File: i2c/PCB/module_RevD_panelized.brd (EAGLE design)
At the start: 100 x 100 mm, 786 parts, among them IC1 ATTINY85-20SU, IC2 ATTINY85-20SU, IC3 ATTINY85-20SU, IC4 ATTINY85-20SU, IC5 ATTINY85-20SU, IC6 ATTINY85-20SU, J1 M20-9980346, J2 M20-9980346, J3 M20-9980346, J4 M20-9980346, J5 M20-9980346, J6 M20-9980346

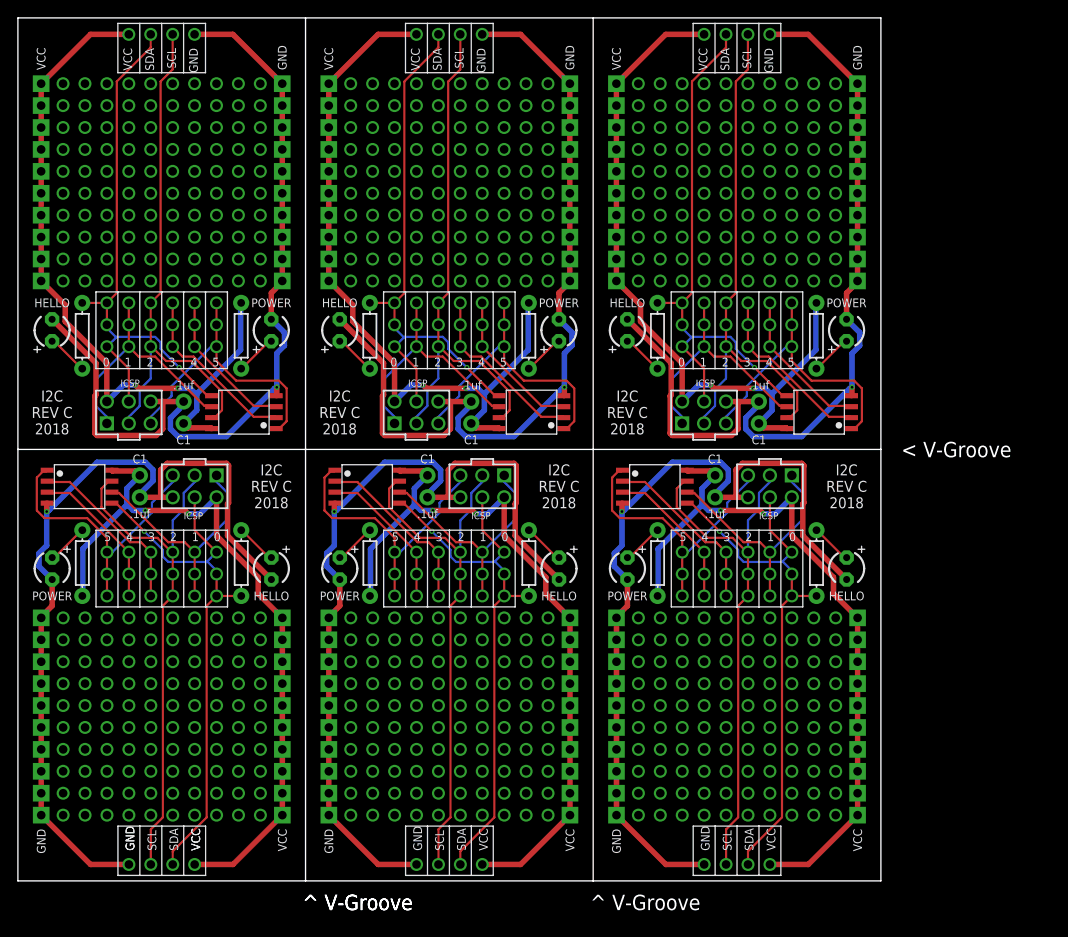
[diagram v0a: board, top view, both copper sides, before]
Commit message: Rework of revD boards
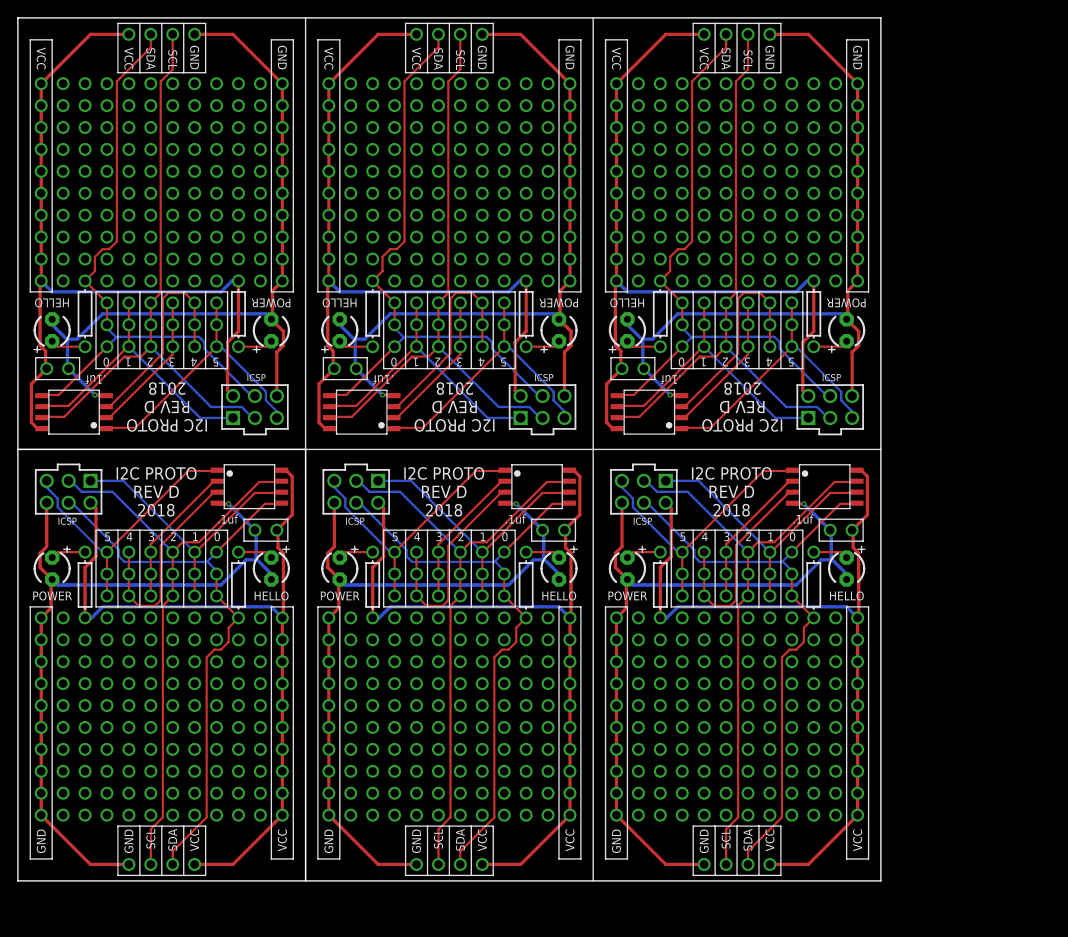
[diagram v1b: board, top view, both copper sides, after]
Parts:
- removed GND, GND1, GND2, GND3, GND4, GND5, VCC, VCC1, VCC2, VCC3, VCC4, VCC5: 10X-PADS, BadgeParts:10X-PADS
- removed R1, R10, R11, R12, R2, R3, R4, R5, R6, R7, R8, R9: 220, SparkFun-Resistors:AXIAL-0.3
- added U$739, U$740, U$741, U$742, U$743, U$744, U$745, U$746, U$747, U$748, U$749, U$750, U$751, U$752, U$753, U$754, U$755, U$756, U$757, U$758, U$759, U$760, U$761, U$762, U$763, U$764, U$765, U$766, U$767, U$768, U$769, U$770, U$771, U$772, U$773, U$774, U$775, U$776, U$777, U$778, U$779, U$780, U$781, U$782, U$783, U$784, U$785, U$790, U$791, U$792, U$793, U$794, U$795, U$796, U$797, U$798, U$799, U$800, U$801, U$802, U$803, U$804, U$805, U$806, U$807, U$808, U$809, U$810, U$811, U$812, U$813, U$814, U$815, U$816, U$817, U$818, U$819, U$820, U$821, U$822, U$823, U$824, U$825, U$826, U$827, U$828, U$829, U$830, U$831, U$832, U$833, U$834, U$835, U$839, U$840, U$841, U$842, U$843, U$844, U$845, U$846, U$847, U$848, U$849, U$850, U$851, U$852, U$853, U$854, U$855, U$856, U$857, U$858: ONE_PAD, BadgeParts:1X01
- added U$786: GND, BadgeParts:1X01
- added U$787: VCC, BadgeParts:1X01
- added U$788: SDA, BadgeParts:1X01
- added U$789: SCL, BadgeParts:1X01
- added U$836: DECOUPLING_CAP, BadgeParts:DECOUPLING_CAP
- added U$837, U$838: RESISTOR, BadgeParts:AXIAL-0.3
- U$126, U$127, U$265, U$266, U$408, U$409, U$551, U$552, U$694, U$695: value ONE_PAD -> RESISTOR; device BadgeParts:1X01 -> BadgeParts:AXIAL-0.3
- U$194, U$317, U$440, U$563, U$686: value GND -> ONE_PAD
- U$195, U$318, U$441, U$564, U$687: value VCC -> ONE_PAD
- U$196, U$319, U$442, U$565, U$688: value SDA -> ONE_PAD
- U$197, U$320, U$443, U$566, U$689: value SCL -> ONE_PAD
- U$214, U$357, U$500, U$643: value ONE_PAD -> GND
- U$215, U$358, U$501, U$644: value ONE_PAD -> VCC
- U$216, U$359, U$502, U$645: value ONE_PAD -> SDA
- U$217, U$360, U$503, U$646: value ONE_PAD -> SCL
- U$246, U$369, U$492, U$615, U$738: value DECOUPLING_CAP -> ONE_PAD; device BadgeParts:DECOUPLING_CAP -> BadgeParts:1X01
- U$264, U$407, U$550, U$693: value ONE_PAD -> DECOUPLING_CAP; device BadgeParts:1X01 -> BadgeParts:DECOUPLING_CAP
- moved U$428 121.6 mm to (97.3, 7.62), turned to 0 degrees
- moved U$424 116.1 mm to (97.3, 12.7), turned to 0 degrees
- moved U$426 111.8 mm to (97.3, 10.2), turned to 0 degrees
- moved U$420 111.0 mm to (97.3, 17.8), turned to 0 degrees
- moved U$422 110.7 mm to (97.3, 15.2), turned to 0 degrees
- moved U$425 109.8 mm to (97.3, 25.4), turned to 0 degrees
- moved U$429 107.4 mm to (97.3, 20.3), turned to 0 degrees
- moved U$427 106.9 mm to (97.3, 22.9), turned to 0 degrees
- moved U$421 105.3 mm to (97.3, 30.5), turned to 0 degrees
- moved U$71 104.5 mm to (12.9, 1.91), turned to 180 degrees
- moved U$423 104.2 mm to (97.3, 27.9), turned to 0 degrees
- moved U$73 102.7 mm to (15.4, 1.91), turned to 0 degrees
- moved U$8 101.7 mm to (5.24, 7.62), turned to 0 degrees
- moved U$72 101.0 mm to (17.9, 1.91), turned to 0 degrees
- moved U$74 99.6 mm to (20.5, 1.91), turned to 90 degrees
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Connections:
- removed net GND4: GND4.P$1, GND4.P$10, GND4.P$2, GND4.P$3, GND4.P$4, GND4.P$5, GND4.P$6, GND4.P$7, GND4.P$8, GND4.P$9, HELLO4.NEG, IC5.GND, J5.GND, POWER4.NEG, U$563.P$1, U$615.1
- removed net GND5: GND5.P$1, GND5.P$10, GND5.P$2, GND5.P$3, GND5.P$4, GND5.P$5, GND5.P$6, GND5.P$7, GND5.P$8, GND5.P$9, HELLO5.NEG, IC6.GND, J6.GND, POWER5.NEG, U$686.P$1, U$738.1
- removed net PB28: IC5.PB5, J5.5/RST, U$582.P$1, U$583.P$1, U$584.P$1
- removed net PB29: IC5.PB1, J5.1/MISO, U$570.P$1, U$571.P$1, U$572.P$1
- removed net PB34: IC6.PB5, J6.5/RST, U$705.P$1, U$706.P$1, U$707.P$1
- removed net PB35: IC6.PB1, J6.1/MISO, U$693.P$1, U$694.P$1, U$695.P$1
- new net GND6: HELLO4.NEG, IC5.GND, J5.GND, POWER4.NEG, U$643.P$1, U$693.P$1, U$696.P$1, U$697.P$1, U$698.P$1, U$699.P$1, U$700.P$1, U$701.P$1, U$702.P$1, U$703.P$1, U$704.P$1, U$705.P$1
- new net GND7: HELLO5.NEG, IC6.GND, J6.GND, POWER5.NEG, U$786.P$1, U$836.P$1, U$839.P$1, U$840.P$1, U$841.P$1, U$842.P$1, U$843.P$1, U$844.P$1, U$845.P$1, U$846.P$1, U$847.P$1, U$848.P$1
- new net PB36: IC6.PB4, U$802.P$1, U$803.P$1, U$804.P$1
- new net PB37: IC6.PB2, J6.2/SCK/SCL, U$789.P$1, U$796.P$1, U$797.P$1, U$798.P$1
- new net PB38: IC6.PB5, J6.5/RST, U$805.P$1, U$806.P$1, U$807.P$1
- new net PB39: IC6.PB1, J6.1/MISO, U$793.P$1, U$794.P$1, U$795.P$1
- net GND: now also U$100.P$1, U$123.P$1, U$124.P$1, U$125.P$1, U$128.P$1, U$129.P$1, U$130.P$1, U$131.P$1, U$132.P$1, U$133.P$1, U$99.P$1; no longer GND.P$1, GND.P$10, GND.P$2, GND.P$3, GND.P$4, GND.P$5, GND.P$6, GND.P$7, GND.P$8, GND.P$9, U$123.1
- net GND1: now also U$214.P$1, U$264.P$1, U$267.P$1, U$268.P$1, U$269.P$1, U$270.P$1, U$271.P$1, U$272.P$1, U$273.P$1, U$274.P$1, U$275.P$1, U$276.P$1; no longer GND1.P$1, GND1.P$10, GND1.P$2, GND1.P$3, GND1.P$4, GND1.P$5, GND1.P$6, GND1.P$7, GND1.P$8, GND1.P$9, U$194.P$1, U$246.1
- net GND2: now also U$357.P$1, U$407.P$1, U$410.P$1, U$411.P$1, U$412.P$1, U$413.P$1, U$414.P$1, U$415.P$1, U$416.P$1, U$417.P$1, U$418.P$1, U$419.P$1; no longer GND2.P$1, GND2.P$10, GND2.P$2, GND2.P$3, GND2.P$4, GND2.P$5, GND2.P$6, GND2.P$7, GND2.P$8, GND2.P$9, U$317.P$1, U$369.1
- net GND3: now also U$500.P$1, U$550.P$1, U$553.P$1, U$554.P$1, U$555.P$1, U$556.P$1, U$557.P$1, U$558.P$1, U$559.P$1, U$560.P$1, U$561.P$1, U$562.P$1; no longer GND3.P$1, GND3.P$10, GND3.P$2, GND3.P$3, GND3.P$4, GND3.P$5, GND3.P$6, GND3.P$7, GND3.P$8, GND3.P$9, U$440.P$1, U$492.1
- net N$1: now also U$126.P$3; no longer R1.P$1
- net N$10: now also U$695.P$3; no longer R10.P$1
- net N$11: now also U$837.P$3; no longer R11.P$1
- net N$12: now also U$838.P$3; no longer R12.P$1
- net N$2: now also HELLO.POS, U$127.P$3; no longer POWER1.POS, R3.P$1
- net N$3: now also POWER1.POS, U$265.P$3; no longer HELLO.POS, R2.P$1
- net N$4: now also U$266.P$3; no longer R4.P$1
- net N$5: now also U$408.P$3; no longer R5.P$1
- net N$6: now also U$409.P$3; no longer R6.P$1
- net N$7: now also U$551.P$3; no longer R7.P$1
- net N$8: now also U$552.P$3; no longer R8.P$1
- net N$9: now also U$694.P$3; no longer R9.P$1
- net PB0: now also U$127.P$4; no longer R2.P$2
- net PB10: now also U$233.P$1, U$234.P$1, U$235.P$1; no longer U$213.P$1, U$214.P$1, U$215.P$1
- net PB11: now also U$221.P$1, U$222.P$1, U$223.P$1; no longer U$201.P$1, U$202.P$1, U$203.P$1
- net PB12: now also U$359.P$1, U$361.P$1, U$362.P$1, U$363.P$1, U$409.P$4; no longer R6.P$2, U$319.P$1, U$321.P$1, U$322.P$1, U$323.P$1
- net PB13: now also U$370.P$1, U$371.P$1, U$372.P$1; no longer U$330.P$1, U$331.P$1, U$332.P$1
- net PB14: now also U$373.P$1, U$374.P$1, U$375.P$1; no longer U$333.P$1, U$334.P$1, U$335.P$1
- net PB15: now also U$360.P$1, U$367.P$1, U$368.P$1, U$369.P$1; no longer U$320.P$1, U$327.P$1, U$328.P$1, U$329.P$1
- net PB16: now also U$376.P$1, U$377.P$1, U$378.P$1; no longer U$336.P$1, U$337.P$1, U$338.P$1
- net PB17: now also U$364.P$1, U$365.P$1, U$366.P$1; no longer U$324.P$1, U$325.P$1, U$326.P$1
- net PB18: now also U$502.P$1, U$504.P$1, U$505.P$1, U$506.P$1, U$552.P$4; no longer R8.P$2, U$442.P$1, U$444.P$1, U$445.P$1, U$446.P$1
- net PB19: now also U$513.P$1, U$514.P$1, U$515.P$1; no longer U$453.P$1, U$454.P$1, U$455.P$1
- net PB20: now also U$516.P$1, U$517.P$1, U$518.P$1; no longer U$456.P$1, U$457.P$1, U$458.P$1
- net PB21: now also U$503.P$1, U$510.P$1, U$511.P$1, U$512.P$1; no longer U$443.P$1, U$450.P$1, U$451.P$1, U$452.P$1
- net PB22: now also U$519.P$1, U$520.P$1, U$521.P$1; no longer U$459.P$1, U$460.P$1, U$461.P$1
- net PB23: now also U$507.P$1, U$508.P$1, U$509.P$1; no longer U$447.P$1, U$448.P$1, U$449.P$1
- net PB24: now also U$645.P$1, U$647.P$1, U$648.P$1, U$649.P$1, U$695.P$4; no longer R10.P$2, U$565.P$1, U$567.P$1, U$568.P$1, U$569.P$1
- net PB25: now also U$656.P$1, U$657.P$1, U$658.P$1; no longer U$576.P$1, U$577.P$1, U$578.P$1
- net PB26: now also U$659.P$1, U$660.P$1, U$661.P$1; no longer U$579.P$1, U$580.P$1, U$581.P$1
- net PB27: now also U$646.P$1, U$653.P$1, U$654.P$1, U$655.P$1; no longer U$566.P$1, U$573.P$1, U$574.P$1, U$575.P$1
- net PB30: now also IC5.PB5, J5.5/RST, U$662.P$1, U$663.P$1, U$664.P$1; no longer IC6.PB0, J6.0/MOSI/SDA, R12.P$2, U$688.P$1, U$690.P$1, U$691.P$1, U$692.P$1
- net PB31: now also IC5.PB1, J5.1/MISO, U$650.P$1, U$651.P$1, U$652.P$1; no longer IC6.PB3, U$699.P$1, U$700.P$1, U$701.P$1
- net PB32: now also IC6.PB0, J6.0/MOSI/SDA, U$788.P$1, U$790.P$1, U$791.P$1, U$792.P$1, U$838.P$4; no longer IC6.PB4, U$702.P$1, U$703.P$1, U$704.P$1
- net PB33: now also IC6.PB3, U$799.P$1, U$800.P$1, U$801.P$1; no longer IC6.PB2, J6.2/SCK/SCL, U$689.P$1, U$696.P$1, U$697.P$1, U$698.P$1
- net PB6: now also U$216.P$1, U$218.P$1, U$219.P$1, U$220.P$1, U$266.P$4; no longer R4.P$2, U$196.P$1, U$198.P$1, U$199.P$1, U$200.P$1
- net PB7: now also U$227.P$1, U$228.P$1, U$229.P$1; no longer U$207.P$1, U$208.P$1, U$209.P$1
- net PB8: now also U$230.P$1, U$231.P$1, U$232.P$1; no longer U$210.P$1, U$211.P$1, U$212.P$1
- net PB9: now also U$217.P$1, U$224.P$1, U$225.P$1, U$226.P$1; no longer U$197.P$1, U$204.P$1, U$205.P$1, U$206.P$1
- net VCC: now also U$123.P$2, U$126.P$4, U$134.P$1, U$135.P$1, U$136.P$1, U$137.P$1, U$138.P$1, U$139.P$1, U$140.P$1, U$141.P$1, U$142.P$1, U$143.P$1; no longer R1.P$2, U$123.2, VCC.P$1, VCC.P$10, VCC.P$2, VCC.P$3, VCC.P$4, VCC.P$5, VCC.P$6, VCC.P$7, VCC.P$8, VCC.P$9
- net VCC1: now also U$215.P$1, U$264.P$2, U$265.P$4, U$277.P$1, U$278.P$1, U$279.P$1, U$280.P$1, U$281.P$1, U$282.P$1, U$283.P$1, U$284.P$1, U$285.P$1, U$286.P$1; no longer R3.P$2, U$195.P$1, U$246.2, VCC1.P$1, VCC1.P$10, VCC1.P$2, VCC1.P$3, VCC1.P$4, VCC1.P$5, VCC1.P$6, VCC1.P$7, VCC1.P$8, VCC1.P$9
- net VCC2: now also U$358.P$1, U$407.P$2, U$408.P$4, U$420.P$1, U$421.P$1, U$422.P$1, U$423.P$1, U$424.P$1, U$425.P$1, U$426.P$1, U$427.P$1, U$428.P$1, U$429.P$1; no longer R5.P$2, U$318.P$1, U$369.2, VCC2.P$1, VCC2.P$10, VCC2.P$2, VCC2.P$3, VCC2.P$4, VCC2.P$5, VCC2.P$6, VCC2.P$7, VCC2.P$8, VCC2.P$9
- net VCC3: now also U$501.P$1, U$550.P$2, U$551.P$4, U$563.P$1, U$564.P$1, U$565.P$1, U$566.P$1, U$567.P$1, U$568.P$1, U$569.P$1, U$570.P$1, U$571.P$1, U$572.P$1; no longer R7.P$2, U$441.P$1, U$492.2, VCC3.P$1, VCC3.P$10, VCC3.P$2, VCC3.P$3, VCC3.P$4, VCC3.P$5, VCC3.P$6, VCC3.P$7, VCC3.P$8, VCC3.P$9
- net VCC4: now also U$644.P$1, U$693.P$2, U$694.P$4, U$706.P$1, U$707.P$1, U$708.P$1, U$709.P$1, U$710.P$1, U$711.P$1, U$712.P$1, U$713.P$1, U$714.P$1, U$715.P$1; no longer R9.P$2, U$564.P$1, U$615.2, VCC4.P$1, VCC4.P$10, VCC4.P$2, VCC4.P$3, VCC4.P$4, VCC4.P$5, VCC4.P$6, VCC4.P$7, VCC4.P$8, VCC4.P$9
- net VCC5: now also U$787.P$1, U$836.P$2, U$837.P$4, U$849.P$1, U$850.P$1, U$851.P$1, U$852.P$1, U$853.P$1, U$854.P$1, U$855.P$1, U$856.P$1, U$857.P$1, U$858.P$1; no longer R11.P$2, U$687.P$1, U$738.2, VCC5.P$1, VCC5.P$10, VCC5.P$2, VCC5.P$3, VCC5.P$4, VCC5.P$5, VCC5.P$6, VCC5.P$7, VCC5.P$8, VCC5.P$9
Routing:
- net GND4: track 99.7 -> 0.00 mm, vias 1 -> 0
- net GND5: track 99.7 -> 0.00 mm, vias 1 -> 0
- net GND7: track 0.00 -> 87.5 mm, vias 0 -> 1
- net GND6: track 0.00 -> 87.5 mm, vias 0 -> 1
- net PB37: track 0.00 -> 68.8 mm
- net PB32: track 17.4 -> 71.0 mm
- net PB33: track 61.3 -> 16.7 mm
- net PB28: track 34.0 -> 0.00 mm
- net PB34: track 34.0 -> 0.00 mm
- net PB39: track 0.00 -> 33.5 mm
- net PB38: track 0.00 -> 33.2 mm
- net PB30: track 63.8 -> 33.2 mm, vias 1 -> 0
- net PB29: track 28.5 -> 0.00 mm
- net PB35: track 28.5 -> 0.00 mm
- net PB36: track 0.00 -> 25.0 mm
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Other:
- outline, holes or cut-outs redrawn
- board text added: "I2C PROTO REV D 2018"
- board text removed: "C1"
- board text removed: "I2C REV C 2018"
